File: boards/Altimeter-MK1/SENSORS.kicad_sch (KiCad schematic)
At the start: 14 parts, among them U1 LSM9DS1, U2 MS5611-01BA, U3 H3LIS331DL

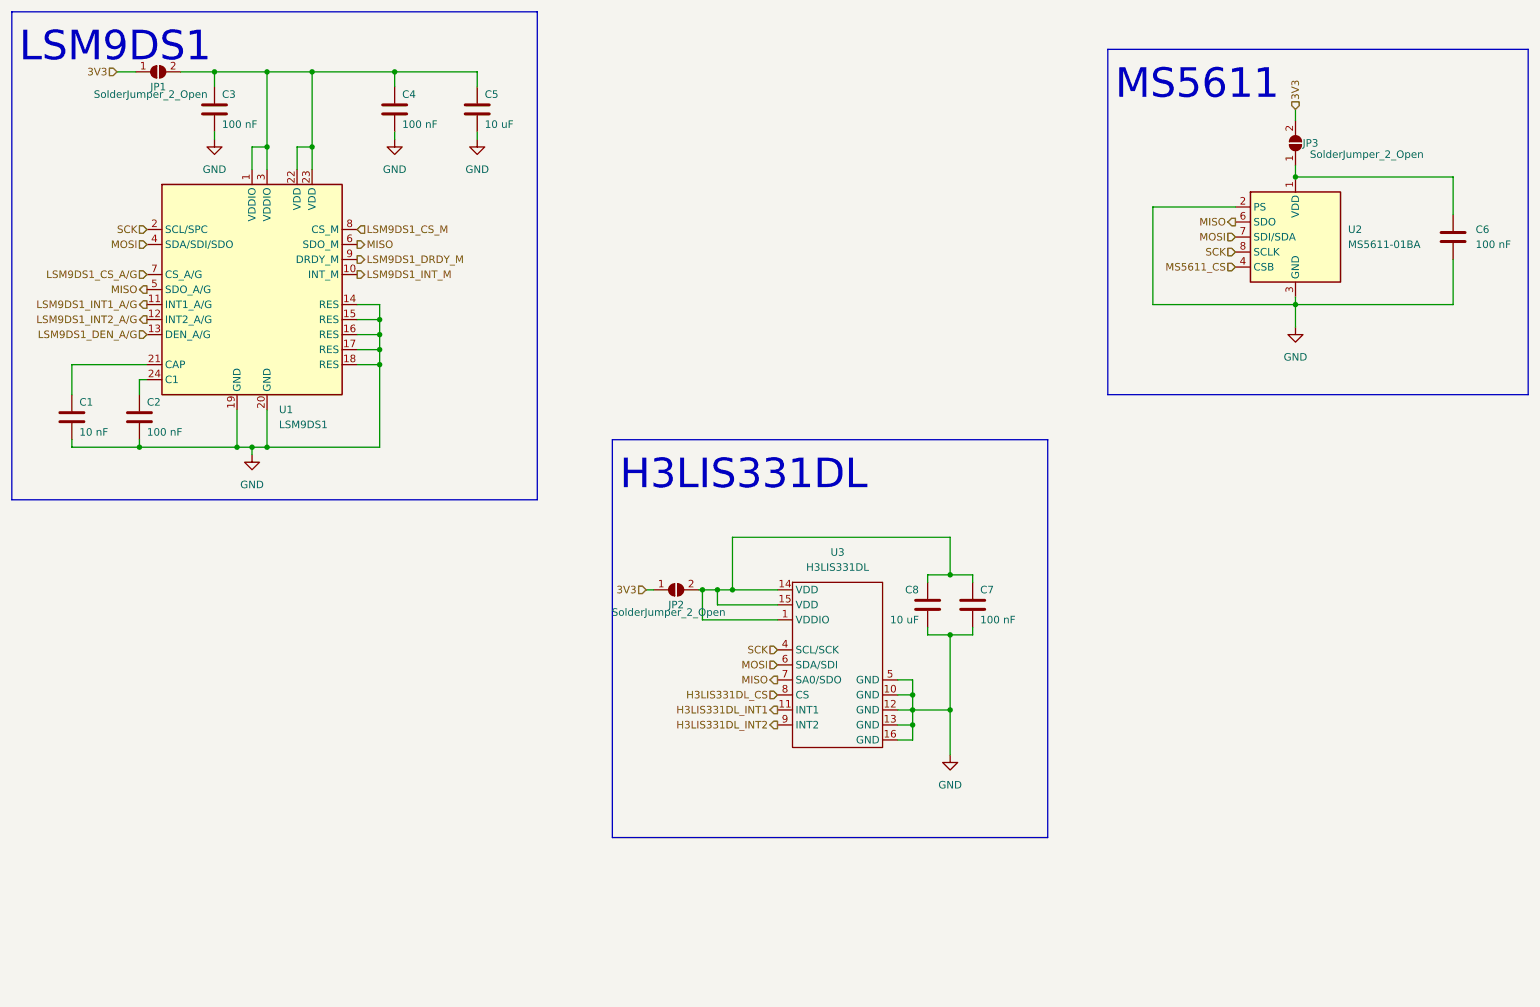
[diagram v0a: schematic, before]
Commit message: Trello not working/mcu sensor connections (#119)
* connected ejection/sensors sheets to mcu

* added gps module to sensor sheet and repositioned boxes (#115)

Co-authored-by: Eisha Peyyeti <eisha.peyyeti@gmail.com>

* deleted GPS kicad_sch

* Av 685/altimeter mcu schematic (#116)

* added jtag connector and fixed power supply

* added memory chip to schematic

* Update MCU.kicad_sch

* Update MCU.kicad_sch

* Update MCU.kicad_sch

* Delete #auto_saved_files#

* Update MCU.kicad_sch

* formatting changes

* kicad changes

* Changes in MCU and SENSORS

NEVER USE SENSORS BRANCH EVER AGAIN LOL

* removed auto saved files

* Update MCU.kicad_sch

* finished mcu schematic

* Added Ematch sensing

* Organized MCU and added CubeMX File

* added notes on unused nand flash signals

* changed buzzer pwm net name to be all caps

* added usb type c receptacle, and esd protection, to schematic

* added test points

* mcu cleanup

* 8/11 Changes

Connected GPS and HopeFM module. Added voltage sensing

Co-authored-by: Arna Bhardwaj <arnabhardwaj@Arnas-MacBook-Air.local>
Co-authored-by: TurtlePhuchka <richeek2@illinois.edu>
Co-authored-by: Peter Giannetos <pg19@illinois.edu>
Co-authored-by: Eisha Peyyeti <eisha.peyyeti@gmail.com>
Co-authored-by: navyasm <108916984+navyasm@users.noreply.github.com>
Co-authored-by: JayBeeRose <109769325+JayBeeRose@users.noreply.github.com>

Co-authored-by: Arna Bhardwaj <arnabhardwaj@Arnas-MacBook-Air.local>
Co-authored-by: Eisha Peyyeti <eisha.peyyeti@gmail.com>
Co-authored-by: TurtlePhuchka <richeek2@illinois.edu>
Co-authored-by: Peter Giannetos <pg19@illinois.edu>
Co-authored-by: navyasm <108916984+navyasm@users.noreply.github.com>
Co-authored-by: JayBeeRose <109769325+JayBeeRose@users.noreply.github.com>
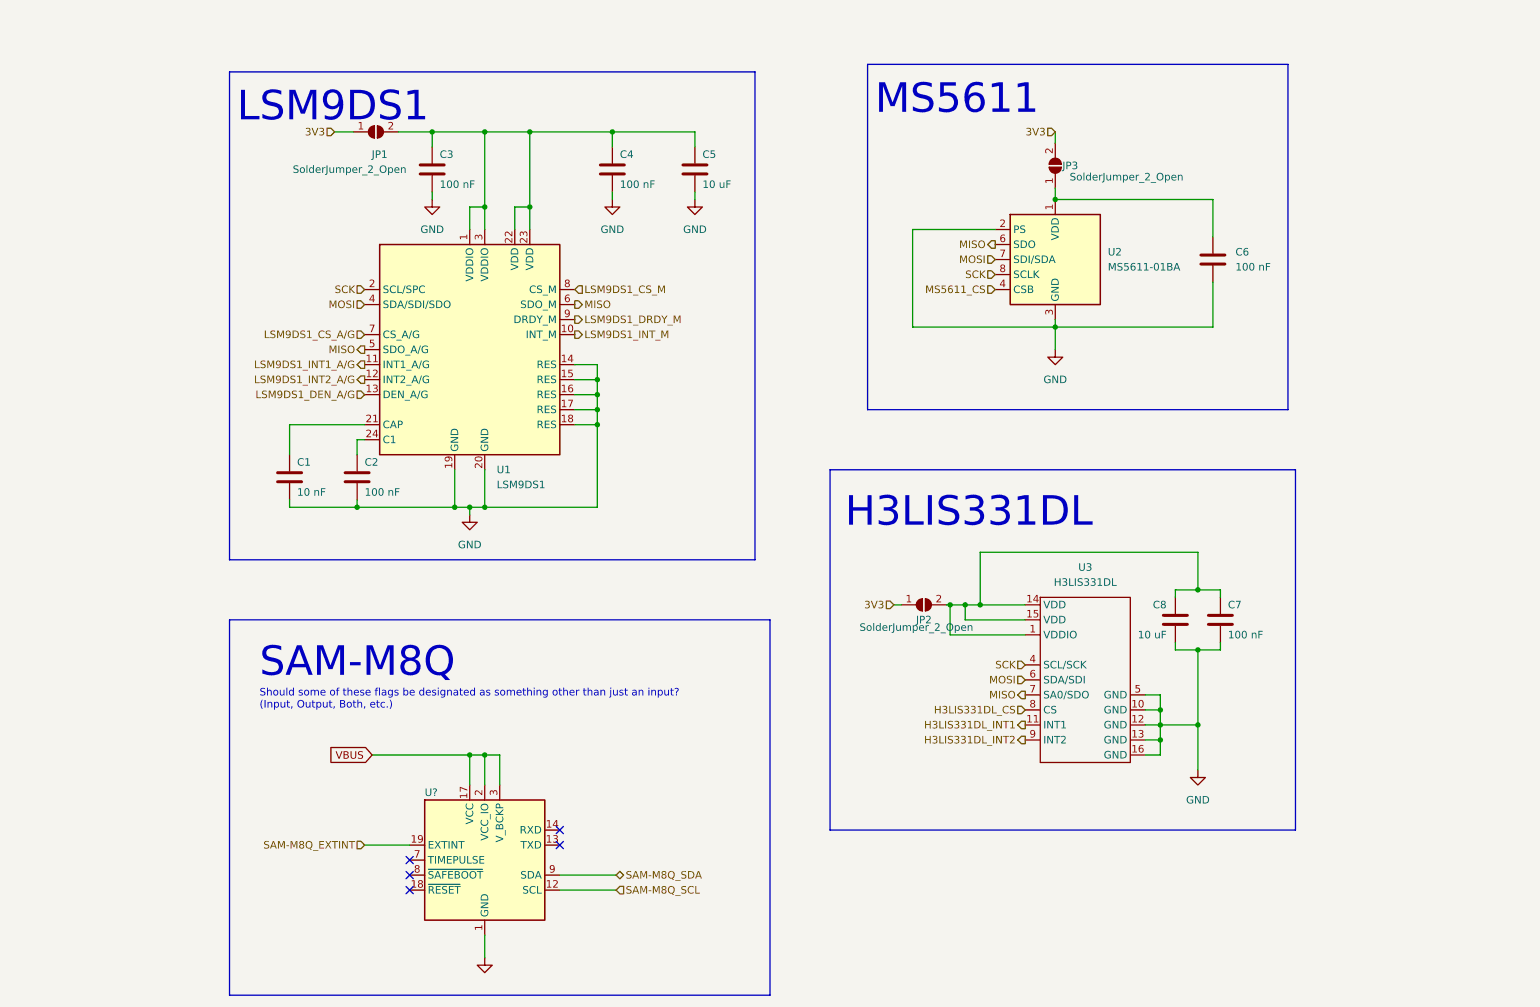
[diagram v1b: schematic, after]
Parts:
- added U?: ~, symbol RF_GPS:SAM-M8Q
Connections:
- net GND: now also U?.1 (GND), U?.10 (GND), U?.11 (GND), U?.15 (GND), U?.16 (GND), U?.20 (GND), U?.4 (GND), U?.5 (GND), U?.6 (GND)
- new net SAM-M8Q_EXTINT: U?.19 (EXTINT)
- new net SAM-M8Q_SCL: U?.12 (SCL)
- new net SAM-M8Q_SDA: U?.9 (SDA)
- new net VBUS: U?.17 (VCC), U?.2 (VCC_IO), U?.3 (V_BCKP)
- no-connect marks 0 -> 5
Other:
- note added: "SAM-M8Q"
- note added: "Should some of these flags be designated as something other than just an input? (Input, Output, Both, etc.)"
- company: (none) -> The Illinois Space Society
- title: (none) -> Altimeter Sensors Schematic Mk1
- moved on the sheet: C1, C2, C3, C4, C5, C6, C7, C8, JP1, JP2, JP3, U1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
